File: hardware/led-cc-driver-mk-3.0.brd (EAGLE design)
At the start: 22.9 x 17.8 mm, 13 parts, among them U1_ ROTARY_ENCODER_SWITCH, U2 Tiny85

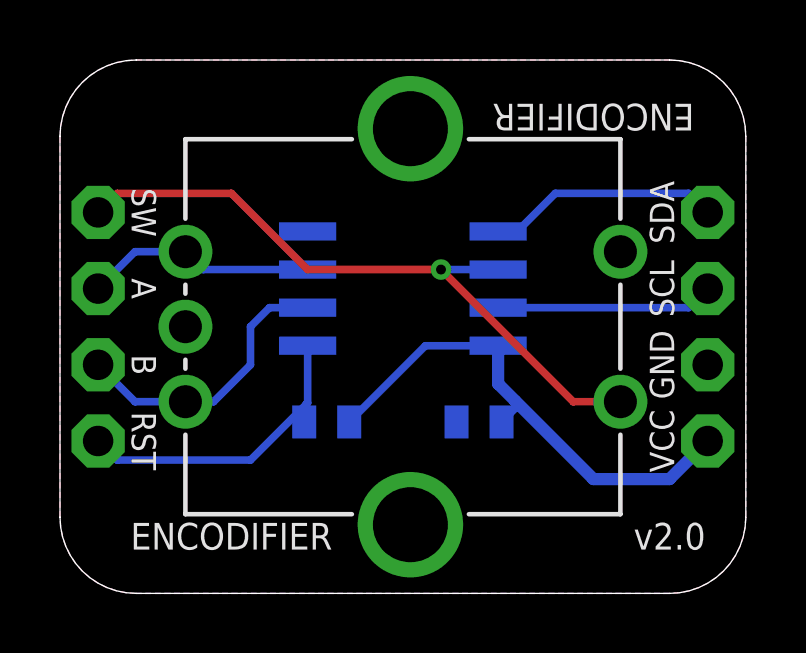
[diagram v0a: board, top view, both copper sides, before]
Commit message: have some boards, dawg
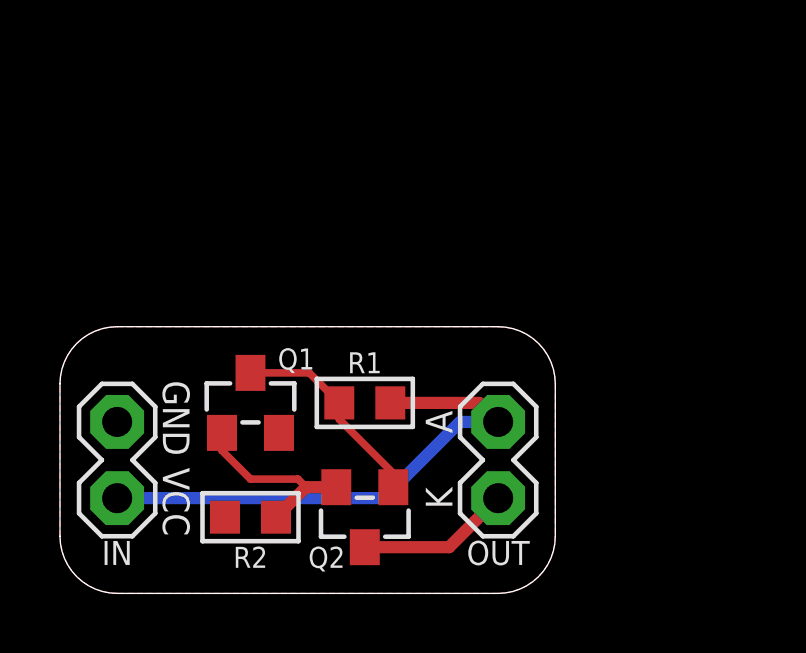
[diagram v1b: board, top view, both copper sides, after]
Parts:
- removed A, B, GND, RST, SCL, SDA, SW, VCC: M01PTH-1MM, a_parts:1X01-1MM-NS
- removed C1: 100n, a_parts:C0603-TIGHTER
- removed U1_: ROTARY_ENCODER_SWITCH, a_parts:ROTARY_ENCODER_SWITCH
- removed U2: Tiny85, a_parts:SO08-EIAJ
- added IN, OUT: M02PTH-CENTERED, a_parts:1X02-CENTER
- added Q1: MMBT2222A, a_parts:SOT23
- added Q2: IRLML2502, a_parts:SOT23
- added R2: Iset, a_parts:R0603
- added U$1: (no value), a_parts:COW_SMALL_NOTEXT
- R1: value 10k -> 100K; device a_parts:R0603-TIGHTER -> a_parts:R0603
- moved R1 1.42 mm to (10.2, 6.35), flipped to the top, turned to 0 degrees
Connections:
- removed net A: A.1, U1_.A, U2.3
- removed net B: B.1, U1_.B, U2.2
- removed net MOSI/SDA: SDA.1, U2.5
- removed net RST: R1.1, RST.1, U2.1
- removed net SCK/SCL: SCL.1, U2.7
- removed net SW: SW.1, U1_.SW1, U2.6
- new net N$1: Q1.3, Q2.1, R1.1
- new net N$2: Q1.1, Q2.2, R2.2
- new net N$4: OUT.1, Q2.3
- net GND: now also IN.1, Q1.2, R2.1; no longer C1.2, GND.1, U1_.C, U1_.SW2, U2.4
- net VCC: now also IN.2, OUT.2; no longer C1.1, U2.8, VCC.1
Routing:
- net SW: track 22.5 -> 0.00 mm, vias 1 -> 0
- net RST: track 10.5 -> 0.00 mm
- net B: track 9.54 -> 0.00 mm
- net MOSI/SDA: track 7.77 -> 0.00 mm
- net A: track 7.74 -> 0.00 mm
- net SCK/SCL: track 7.25 -> 0.00 mm
- net N$1: track 0.00 -> 6.93 mm
- net N$2: track 0.00 -> 6.32 mm
- net N$4: track 0.00 -> 5.12 mm
- net VCC: track 17.0 -> 17.6 mm
- removed copper zone on layer 16, net GND
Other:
- board size 22.9 x 17.8 mm -> 16.5 x 8.9 mm
- board text added: "Constant Current LED Driver"
- board text added: "GND"
- board text added: "K"
- board text added: "VCC"
- board text removed: "B"
- board text removed: "C"
- board text removed: "COM"
- board text removed: "ENCODIFIER"
- board text removed: "SW"
